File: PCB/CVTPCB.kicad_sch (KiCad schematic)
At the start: 13 parts, among them J1 Conn_01x09_Pin, J4 2x1, J7 SystemInput

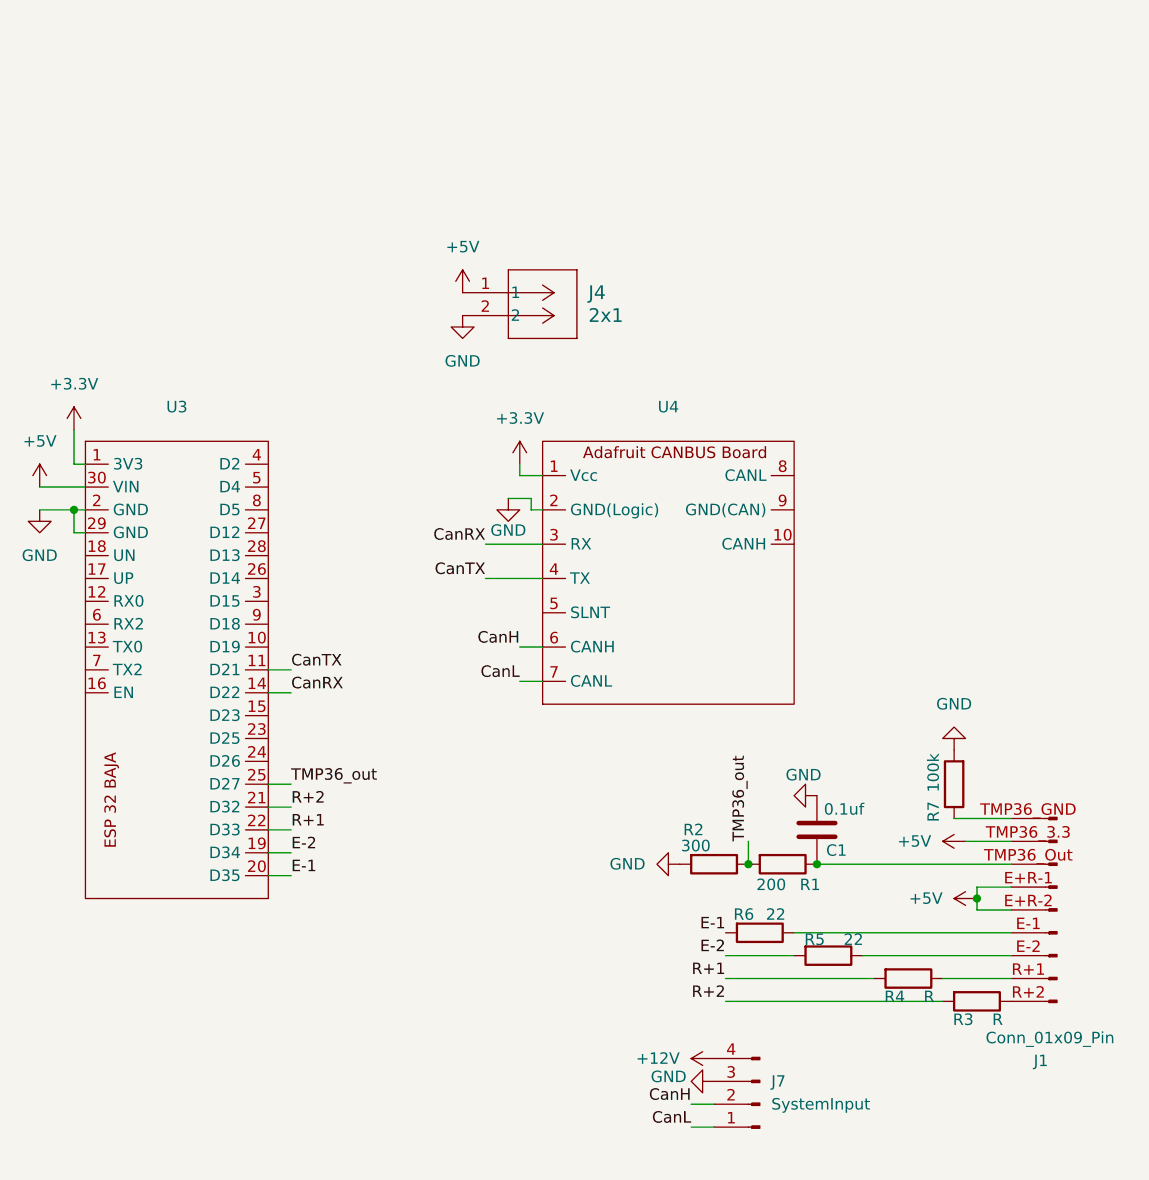
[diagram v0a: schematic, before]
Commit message: Add files via upload
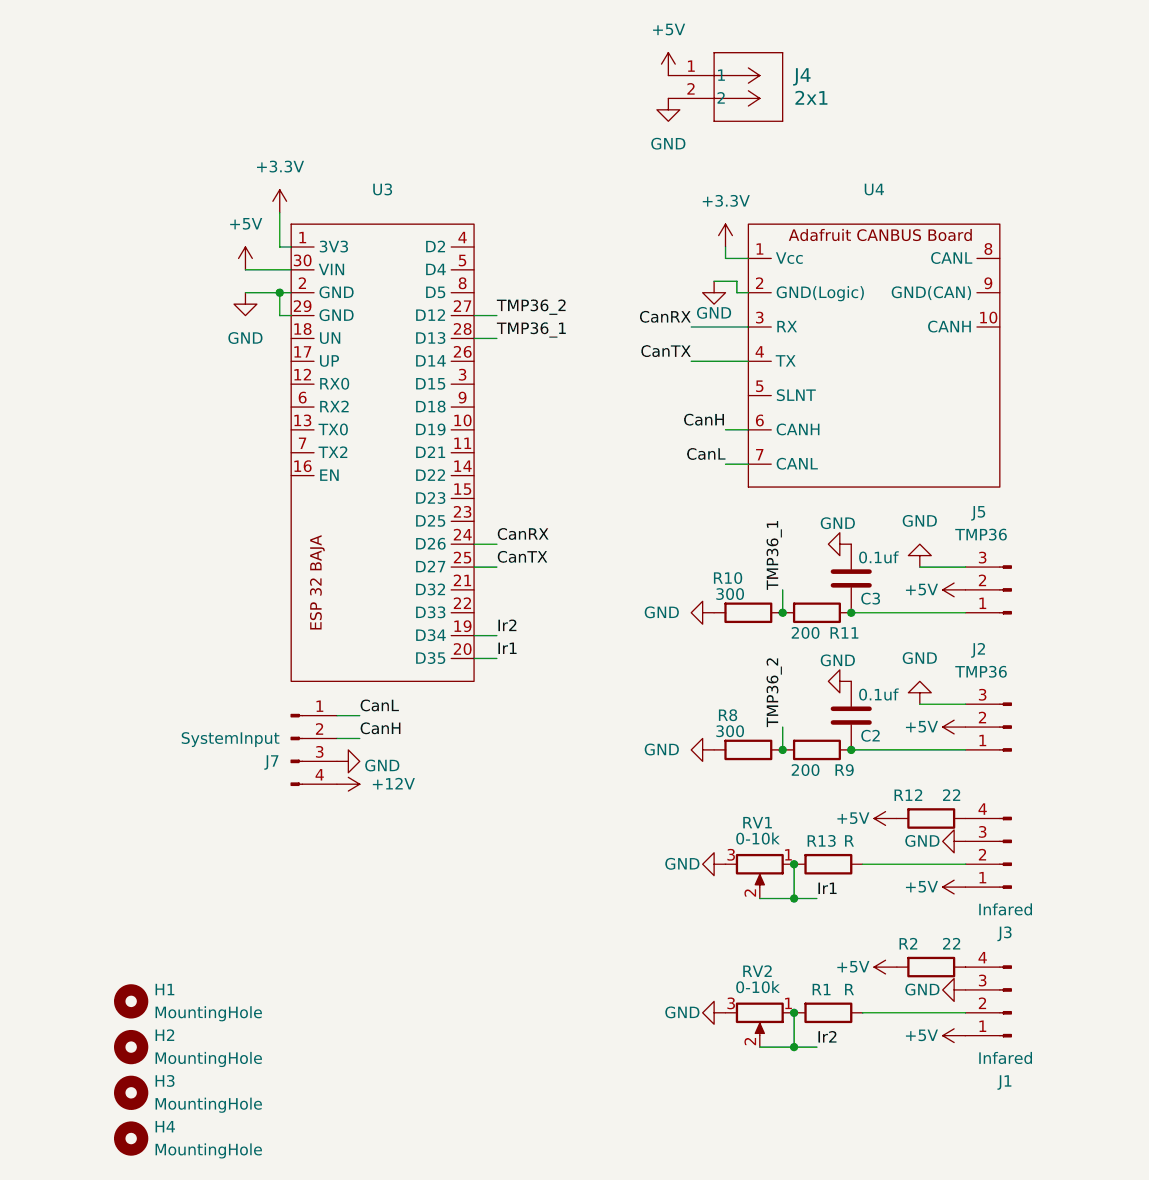
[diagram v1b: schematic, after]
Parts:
- removed C1: 0.1uf, symbol Device:C
- removed J1: Conn_01x09_Pin, symbol Connector:Conn_01x09_Pin
- removed R3, R4: R, symbol Device:R
- removed R5, R6: 22, symbol Device:R
- removed R7: 100k, symbol Device:R
- added C2, C3: 0.1uf, Capacitor_THT:C_Disc_D3.0mm_W2.0mm_P2.50mm, symbol Device:C
- added H1, H2, H3, H4: MountingHole, MountingHole:MountingHole_4.3mm_M4, symbol Mechanical:MountingHole
- added J1, J3: Infared, CVT:Infared, symbol Connector:Conn_01x04_Pin
- added J2, J5: TMP36, CVT:TMP36_Pad, symbol Connector:Conn_01x03_Pin
- added R10, R8: 300, Resistor_THT:R_Axial_DIN0204_L3.6mm_D1.6mm_P5.08mm_Horizontal, symbol Device:R
- added R11, R9: 200, Resistor_THT:R_Axial_DIN0204_L3.6mm_D1.6mm_P5.08mm_Horizontal, symbol Device:R
- added R12: 22, Resistor_THT:R_Axial_DIN0204_L3.6mm_D1.6mm_P5.08mm_Horizontal, symbol Device:R
- added R13: R, Resistor_THT:R_Axial_DIN0204_L3.6mm_D1.6mm_P5.08mm_Horizontal, symbol Device:R
- added RV1, RV2: 0-10k, Potentiometer_THT:Potentiometer_Bourns_3339H_Vertical, symbol Device:R_Potentiometer
- J4: footprint CONN_S2B-PH-K-S_JST -> Connector_PinHeader_1.00mm:PinHeader_1x02_P1.00mm_Vertical
- J7: footprint (none) -> CVT:JST4Pin
- R1: value 200 -> R; footprint (none) -> Resistor_THT:R_Axial_DIN0204_L3.6mm_D1.6mm_P5.08mm_Horizontal
- R2: value 300 -> 22; footprint (none) -> Resistor_THT:R_Axial_DIN0204_L3.6mm_D1.6mm_P5.08mm_Horizontal
- U3: footprint ESP 32:ESP 32 BAJA -> CVT:ESP 32 BAJA
- U4: footprint (none) -> CVT:1x7 Connectors
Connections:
- net +5V: now also R2.2, J1.1 (IR+), J2.2 (3.3+), J3.1 (IR+), J5.2 (3.3+), R12.2
- net CanRX: now also U3.24 (D26); no longer U3.14 (D22)
- net CanTX: now also U3.25 (D27); no longer U3.11 (D21)
- net GND: now also C2.1, C3.1, J1.3 (E-), J2.3 (GND), J3.3 (E-), J5.3 (GND), R10.2, R8.2, RV1.3, RV2.3; no longer R2.2
- net at R1.1: now also J1.2 (IR-)
- net TMP36_2: now reaches U3.27 (D12)
- net TMP36_2: now also R8.1, R9.2
- net TMP36_1: now reaches U3.28 (D13)
- net TMP36_1: now also R10.1, R11.2
- net E-1 renamed Ir1
- net Ir1: now also R13.2, RV1.1, RV1.2
- net E-2 renamed Ir2
- net Ir2: now also R1.2, RV2.1, RV2.2
- net R+1: no longer names the net of U3.22 (D33)
- net R+2: no longer names the net of U3.21 (D32)
- removed net TMP36_out: R1.2, R2.1, U3.25 (D27)
- new net: J3.2 (IR-), R13.1
- new net: J3.4 (E+), R12.1
- new net: J1.4 (E+), R2.1
- new net: C3.2, J5.1 (s), R11.1
- new net: C2.2, J2.1 (s), R9.1
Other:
- moved on the sheet: J4, J7, U3, U4
